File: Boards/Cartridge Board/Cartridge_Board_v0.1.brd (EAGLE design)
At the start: 481.3 x 352.7 mm, 6 parts, among them X1 22-23-2071, X2 22-23-2071

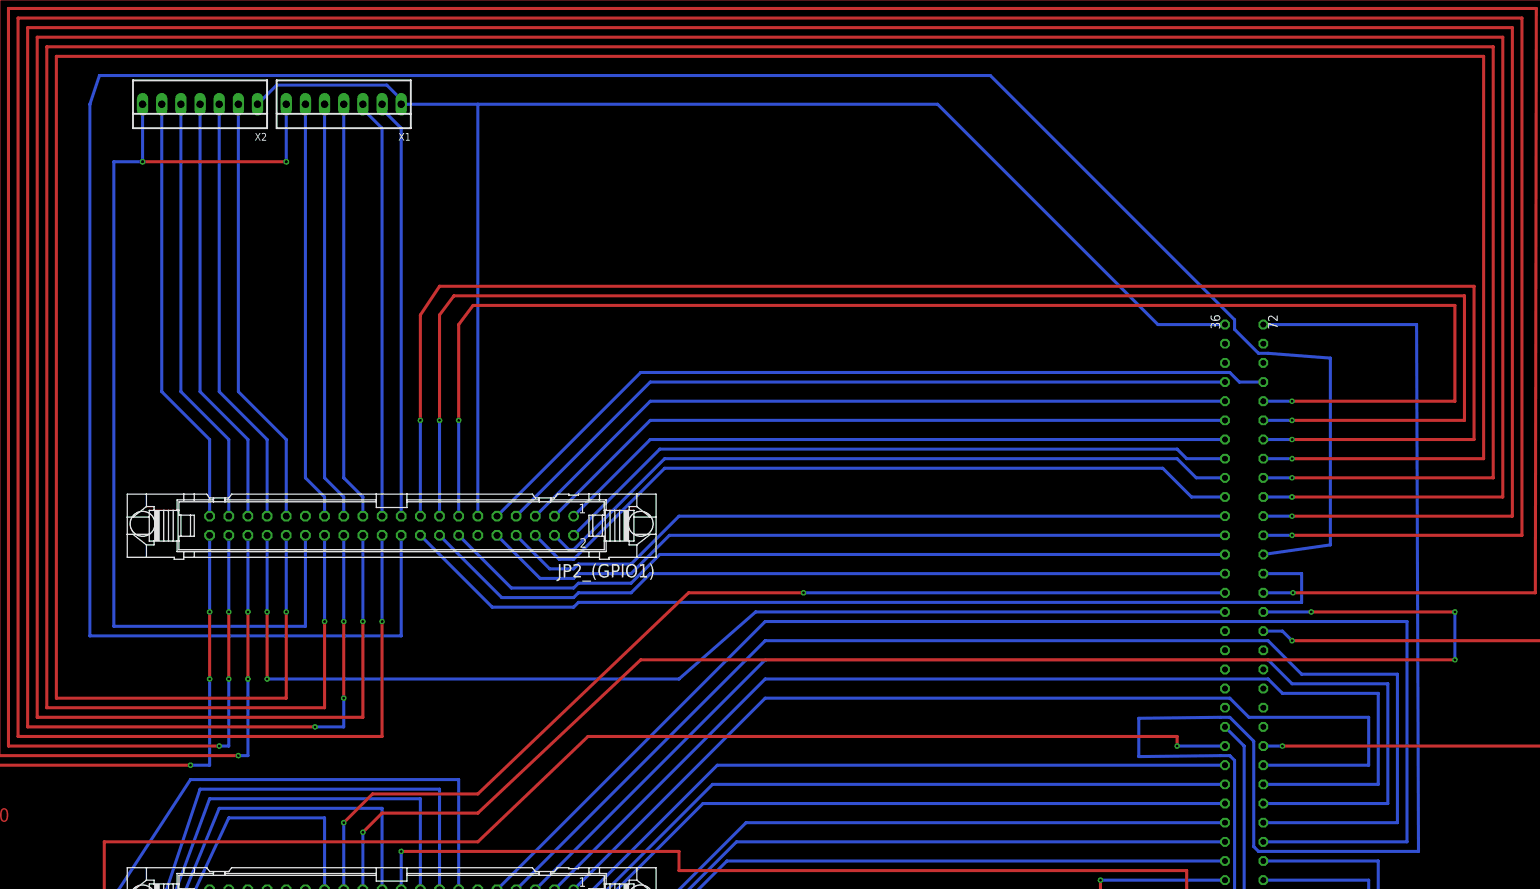
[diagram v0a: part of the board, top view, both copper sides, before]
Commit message: SLoW AnD STEaDY
wins the rase
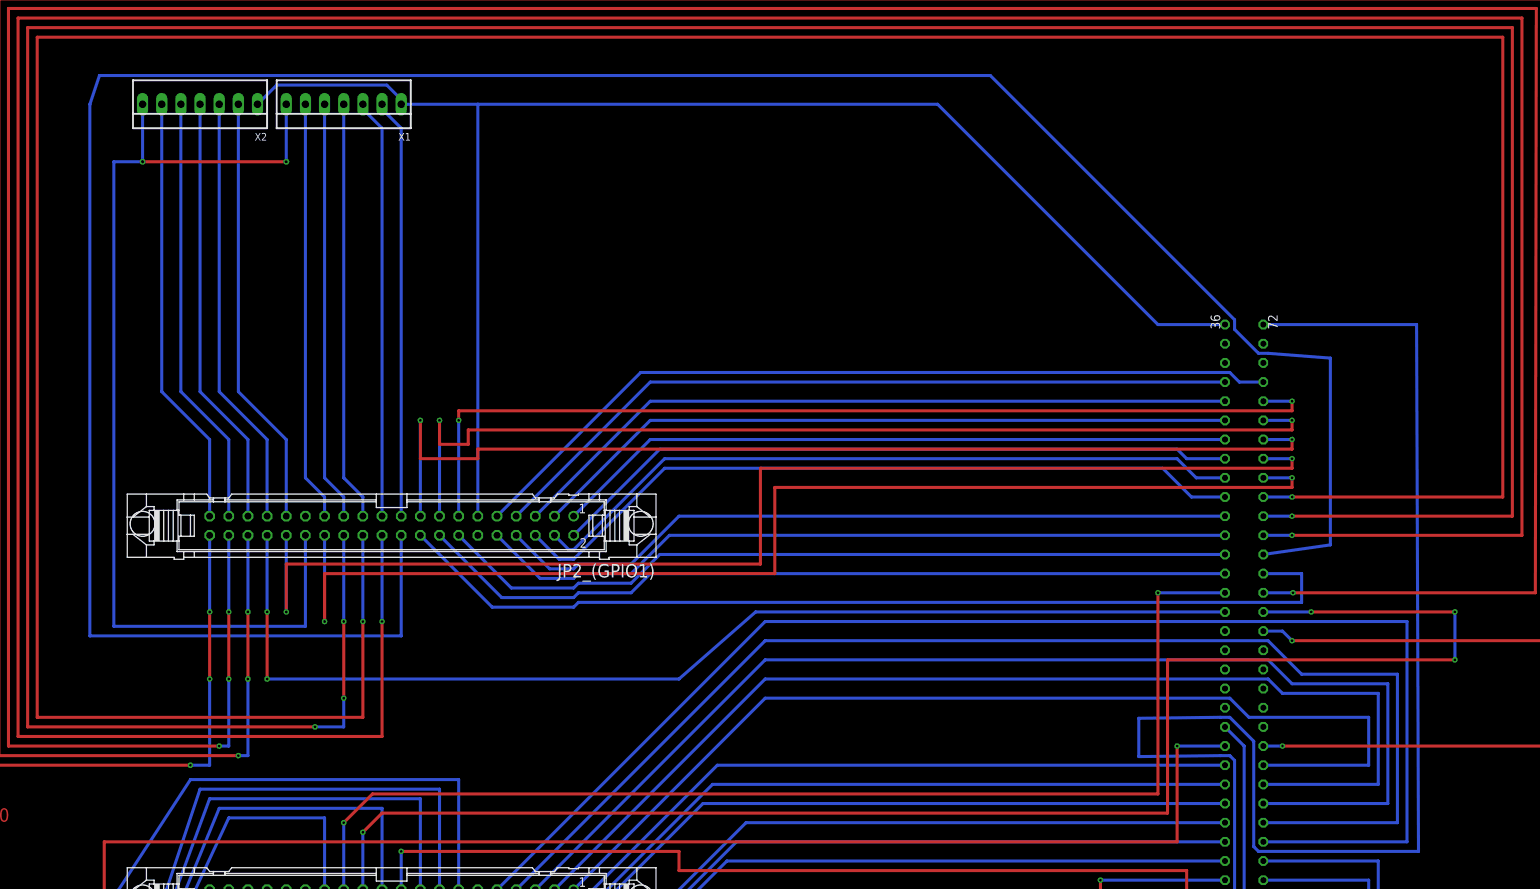
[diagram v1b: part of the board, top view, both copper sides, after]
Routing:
- net PPU_A12: track 426.7 -> 162.6 mm
- net PPU_A13: track 408.9 -> 167.6 mm
- net PPU_D7: track 216.7 -> 139.7 mm
- net PPU_D6: track 207.0 -> 135.9 mm
- net PPU_D5: track 196.9 -> 129.5 mm
- net CIRAM_A10: track 138.0 -> 154.0 mm
- net CIRAM/CE: track 193.3 -> 205.5 mm
- net CPU_R/W: track 198.6 -> 204.5 mm
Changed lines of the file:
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@@
 <setting verticaltext="up"/>
 </settings>
-<grid distance="250" unitdist="mil" unit="mil" style="lines" multiple="1" display="yes" altdistance="5" altunitdist="mil" altunit="mil"/>
+<grid distance="25" unitdist="mil" unit="mil" style="lines" multiple="2" display="yes" altdistance="5" altunitdist="mil" altunit="mil"/>
 <layers>
 <layer number="1" name="Top" color="4" fill="1" visible="yes" active="yes"/>
@@
 <wire x1="144.78" y1="6.35" x2="144.78" y2="0" width="0.4064" layer="16"/>
 <via x="144.78" y="0" extent="1-16" drill="0.35"/>
-<wire x1="36.83" y1="0" x2="15.24" y2="-20.32" width="0.4064" layer="1"/>
-<wire x1="144.78" y1="0" x2="36.83" y2="0" width="0.4064" layer="1"/>
+<wire x1="106.68" y1="0" x2="106.68" y2="-20.32" width="0.4064" layer="1"/>
+<wire x1="144.78" y1="0" x2="106.68" y2="0" width="0.4064" layer="1"/>
 <wire x1="2.54" y1="-20.32" x2="0" y2="-22.86" width="0.4064" layer="1"/>
-<wire x1="15.24" y1="-20.32" x2="2.54" y2="-20.32" width="0.4064" layer="1"/>
+<wire x1="106.68" y1="-20.32" x2="2.54" y2="-20.32" width="0.4064" layer="1"/>
 <via x="0" y="-22.86" extent="1-16" drill="0.35"/>
 <wire x1="0" y1="-22.86" x2="0" y2="-30.48" width="0.4064" layer="16"/>
@@
 <wire x1="119.38" y1="24.13" x2="123.19" y2="24.13" width="0.4064" layer="16"/>
 <via x="123.19" y="24.13" extent="1-16" drill="0.35"/>
-<wire x1="149.86" y1="24.13" x2="149.86" y2="81.28" width="0.4064" layer="1"/>
-<wire x1="149.86" y1="81.28" x2="-41.91" y2="81.28" width="0.4064" layer="1"/>
-<wire x1="-41.91" y1="81.28" x2="-41.91" y2="-6.35" width="0.4064" layer="1"/>
-<wire x1="-41.91" y1="-6.35" x2="-5.08" y2="-6.35" width="0.4064" layer="1"/>
-<wire x1="123.19" y1="24.13" x2="149.86" y2="24.13" width="0.4064" layer="1"/>
-<wire x1="-5.08" y1="-6.35" x2="-5.08" y2="5.08" width="0.4064" layer="1"/>
+<wire x1="123.19" y1="22.86" x2="54.61" y2="22.86" width="0.4064" layer="1"/>
+<wire x1="54.61" y1="22.86" x2="54.61" y2="11.43" width="0.4064" layer="1"/>
+<wire x1="54.61" y1="11.43" x2="-5.08" y2="11.43" width="0.4064" layer="1"/>
+<wire x1="123.19" y1="24.13" x2="123.19" y2="22.86" width="0.4064" layer="1"/>
+<wire x1="-5.08" y1="11.43" x2="-5.08" y2="5.08" width="0.4064" layer="1"/>
 <via x="-5.08" y="5.08" extent="1-16" drill="0.35"/>
 <wire x1="-5.08" y1="5.08" x2="-5.08" y2="16.51" width="0.4064" layer="16"/>
@@
 <wire x1="119.38" y1="26.67" x2="123.19" y2="26.67" width="0.4064" layer="16"/>
 <via x="123.19" y="26.67" extent="1-16" drill="0.35"/>
-<wire x1="123.19" y1="26.67" x2="148.59" y2="26.67" width="0.4064" layer="1"/>
-<wire x1="148.59" y1="26.67" x2="148.59" y2="80.01" width="0.4064" layer="1"/>
-<wire x1="148.59" y1="80.01" x2="-40.64" y2="80.01" width="0.4064" layer="1"/>
-<wire x1="-40.64" y1="80.01" x2="-40.64" y2="-5.08" width="0.4064" layer="1"/>
-<wire x1="-40.64" y1="-5.08" x2="-10.16" y2="-5.08" width="0.4064" layer="1"/>
-<wire x1="-10.16" y1="-5.08" x2="-10.16" y2="6.35" width="0.4064" layer="1"/>
+<wire x1="123.19" y1="26.67" x2="123.19" y2="25.4" width="0.4064" layer="1"/>
+<wire x1="123.19" y1="25.4" x2="52.705" y2="25.4" width="0.4064" layer="1"/>
+<wire x1="52.705" y1="25.4" x2="52.705" y2="12.7" width="0.4064" layer="1"/>
+<wire x1="52.705" y1="12.7" x2="-10.16" y2="12.7" width="0.4064" layer="1"/>
+<wire x1="-10.16" y1="12.7" x2="-10.16" y2="6.35" width="0.4064" layer="1"/>
 <via x="-10.16" y="6.35" extent="1-16" drill="0.35"/>
 <wire x1="-10.16" y1="6.35" x2="-10.16" y2="16.51" width="0.4064" layer="16"/>
@@
 <wire x1="119.38" y1="29.21" x2="123.19" y2="29.21" width="0.4064" layer="16"/>
 <via x="123.19" y="29.21" extent="1-16" drill="0.35"/>
-<wire x1="147.32" y1="29.21" x2="147.32" y2="49.53" width="0.4064" layer="1"/>
-<wire x1="147.32" y1="49.53" x2="10.16" y2="49.53" width="0.4064" layer="1"/>
-<wire x1="10.16" y1="49.53" x2="7.62" y2="45.72" width="0.4064" layer="1"/>
-<wire x1="7.62" y1="45.72" x2="7.62" y2="31.75" width="0.4064" layer="1"/>
-<wire x1="123.19" y1="29.21" x2="147.32" y2="29.21" width="0.4064" layer="1"/>
+<wire x1="123.19" y1="27.94" x2="15.24" y2="27.94" width="0.4064" layer="1"/>
+<wire x1="15.24" y1="27.94" x2="15.24" y2="26.67" width="0.4064" layer="1"/>
+<wire x1="15.24" y1="26.67" x2="7.62" y2="26.67" width="0.4064" layer="1"/>
+<wire x1="7.62" y1="26.67" x2="7.62" y2="31.75" width="0.4064" layer="1"/>
+<wire x1="123.19" y1="29.21" x2="123.19" y2="27.94" width="0.4064" layer="1"/>
 <via x="7.62" y="31.75" extent="1-16" drill="0.35"/>
 <wire x1="7.62" y1="31.75" x2="7.62" y2="19.05" width="0.4064" layer="16"/>
@@
 <contactref element="U$1" pad="CIRAM_A10"/>
 <contactref element="J1_(GPIO0)" pad="25"/>
-<wire x1="114.3" y1="8.89" x2="58.42" y2="8.89" width="0.4064" layer="16"/>
-<via x="58.42" y="8.89" extent="1-16" drill="0.35"/>
-<wire x1="43.18" y1="8.89" x2="15.24" y2="-17.78" width="0.4064" layer="1"/>
-<wire x1="58.42" y1="8.89" x2="43.18" y2="8.89" width="0.4064" layer="1"/>
-<wire x1="15.24" y1="-17.78" x2="1.27" y2="-17.78" width="0.4064" layer="1"/>
+<wire x1="114.3" y1="8.89" x2="105.41" y2="8.89" width="0.4064" layer="16"/>
+<via x="105.41" y="8.89" extent="1-16" drill="0.35"/>
+<wire x1="105.41" y1="-17.78" x2="1.27" y2="-17.78" width="0.4064" layer="1"/>
+<wire x1="105.41" y1="8.89" x2="105.41" y2="-17.78" width="0.4064" layer="1"/>
 <wire x1="1.27" y1="-17.78" x2="-2.54" y2="-21.59" width="0.4064" layer="1"/>
 <via x="-2.54" y="-21.59" extent="1-16" drill="0.35"/>
@@
 <wire x1="119.38" y1="31.75" x2="123.19" y2="31.75" width="0.4064" layer="16"/>
 <via x="123.19" y="31.75" extent="1-16" drill="0.35"/>
-<wire x1="123.19" y1="31.75" x2="146.05" y2="31.75" width="0.4064" layer="1"/>
-<wire x1="146.05" y1="31.75" x2="146.05" y2="48.26" width="0.4064" layer="1"/>
-<wire x1="146.05" y1="48.26" x2="12.065" y2="48.26" width="0.4064" layer="1"/>
-<wire x1="12.065" y1="48.26" x2="10.16" y2="45.72" width="0.4064" layer="1"/>
-<wire x1="10.16" y1="45.72" x2="10.16" y2="31.75" width="0.4064" layer="1"/>
+<wire x1="123.19" y1="31.75" x2="123.19" y2="30.48" width="0.4064" layer="1"/>
+<wire x1="123.19" y1="30.48" x2="13.97" y2="30.48" width="0.4064" layer="1"/>
+<wire x1="13.97" y1="30.48" x2="13.97" y2="28.575" width="0.4064" layer="1"/>
+<wire x1="13.97" y1="28.575" x2="10.16" y2="28.575" width="0.4064" layer="1"/>
+<wire x1="10.16" y1="28.575" x2="10.16" y2="31.75" width="0.4064" layer="1"/>
 <via x="10.16" y="31.75" extent="1-16" drill="0.35"/>
 <wire x1="10.16" y1="31.75" x2="10.16" y2="19.05" width="0.4064" layer="16"/>
@@
 <wire x1="119.38" y1="34.29" x2="123.19" y2="34.29" width="0.4064" layer="16"/>
 <via x="123.19" y="34.29" extent="1-16" drill="0.35"/>
-<wire x1="123.19" y1="34.29" x2="144.78" y2="34.29" width="0.4064" layer="1"/>
-<wire x1="144.78" y1="34.29" x2="144.78" y2="46.99" width="0.4064" layer="1"/>
-<wire x1="144.78" y1="46.99" x2="14.605" y2="46.99" width="0.4064" layer="1"/>
-<wire x1="14.605" y1="46.99" x2="12.7" y2="44.45" width="0.4064" layer="1"/>
-<wire x1="12.7" y1="44.45" x2="12.7" y2="31.75" width="0.4064" layer="1"/>
+<wire x1="123.19" y1="34.29" x2="123.19" y2="33.02" width="0.4064" layer="1"/>
+<wire x1="123.19" y1="33.02" x2="12.7" y2="33.02" width="0.4064" layer="1"/>
+<wire x1="12.7" y1="33.02" x2="12.7" y2="31.75" width="0.4064" layer="1"/>
 <via x="12.7" y="31.75" extent="1-16" drill="0.35"/>
 <wire x1="12.7" y1="31.75" x2="12.7" y2="19.05" width="0.4064" layer="16"/>
@@
 <contactref element="U$1" pad="CPU_R/W"/>
 <wire x1="114.3" y1="-11.43" x2="107.95" y2="-11.43" width="0.4064" layer="16"/>
-<wire x1="107.95" y1="-11.43" x2="107.95" y2="-10.16" width="0.4064" layer="1"/>
+<wire x1="107.95" y1="-11.43" x2="109.855" y2="-8.89" width="0" layer="19" extent="1-16"/>
 <via x="107.95" y="-11.43" extent="1-16" drill="0.35"/>
-<wire x1="107.95" y1="-10.16" x2="29.845" y2="-10.16" width="0.4064" layer="1"/>
-<wire x1="29.845" y1="-10.16" x2="15.24" y2="-24.13" width="0.4064" layer="1"/>
-<wire x1="15.24" y1="-24.13" x2="-34.29" y2="-24.13" width="0.4064" layer="1"/>
+<wire x1="107.95" y1="-11.43" x2="107.95" y2="-24.13" width="0.4064" layer="1"/>
+<wire x1="107.95" y1="-24.13" x2="-34.29" y2="-24.13" width="0.4064" layer="1"/>
 <wire x1="-34.29" y1="-24.13" x2="-34.29" y2="-40.64" width="0.4064" layer="1"/>
 <wire x1="-34.29" y1="-40.64" x2="-15.24" y2="-40.64" width="0.4064" layer="1"/>
